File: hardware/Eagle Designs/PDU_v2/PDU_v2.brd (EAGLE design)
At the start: 90.2 x 95.5 mm, 259 parts, among them J1 5037630291, J10 5037630691, J11 UJ31-CH-G1-SMT-TR, J13 5037630291, J14 5037630291, J16 5037630291, J17 5037630291, J18 5037630491, J19 5037630491, J2 5037630291, J20 503182-1852, J21 5037630491, J26 1729128, J29 61300411021, J3 5037630291, J4 5037630291, J5 5037630291, J6 5037630291, J7 5037630491, J8 5037630491, J9 5037630491, M1 BSZ100N06LS3, M2 BSZ100N06LS3, M3 BSZ033NE2LS5, M4 BSZ033NE2LS5, Q1 FDS6375, Q2 FDS6375, Q3 AO4485, SW1 KMR231GLFS, U1 DRV8847PWPR, U11 IRLML2803PBFCT-ND, U12 IRLML2803PBFCT-ND, U13 LT8390EFE#PBF, U14 ATSAME51N19A-AF, U15 INA219BIDR, U16 MAX706RESA+T, U17 MAX16998AAUA+T, U18 ADT7311WTRZ, U19 NTGD1100LT1G, U2 DRV8847PWPR, U20 AO3404A, U21 LT8609A, U22 LT8609A, U23 BC848ALT1G, U3 LTC1477CS8LINEAR_TECHNOLOGY_L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, U4 LTC1477CS8LINEAR_TECHNOLOGY_L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, U5 LTC1477CS8LINEAR_TECHNOLOGY_L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, U6 LTC1477CS8LINEAR_TECHNOLOGY_L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, U7 LTC1477CS8LINEAR_TECHNOLOGY_L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, U8 LT8609A, U9 LTC1477CS8LINEAR_TECHNOLOGY_L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, Y1 CC4V-T1A-32.768KHZ-12.5PF-20P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

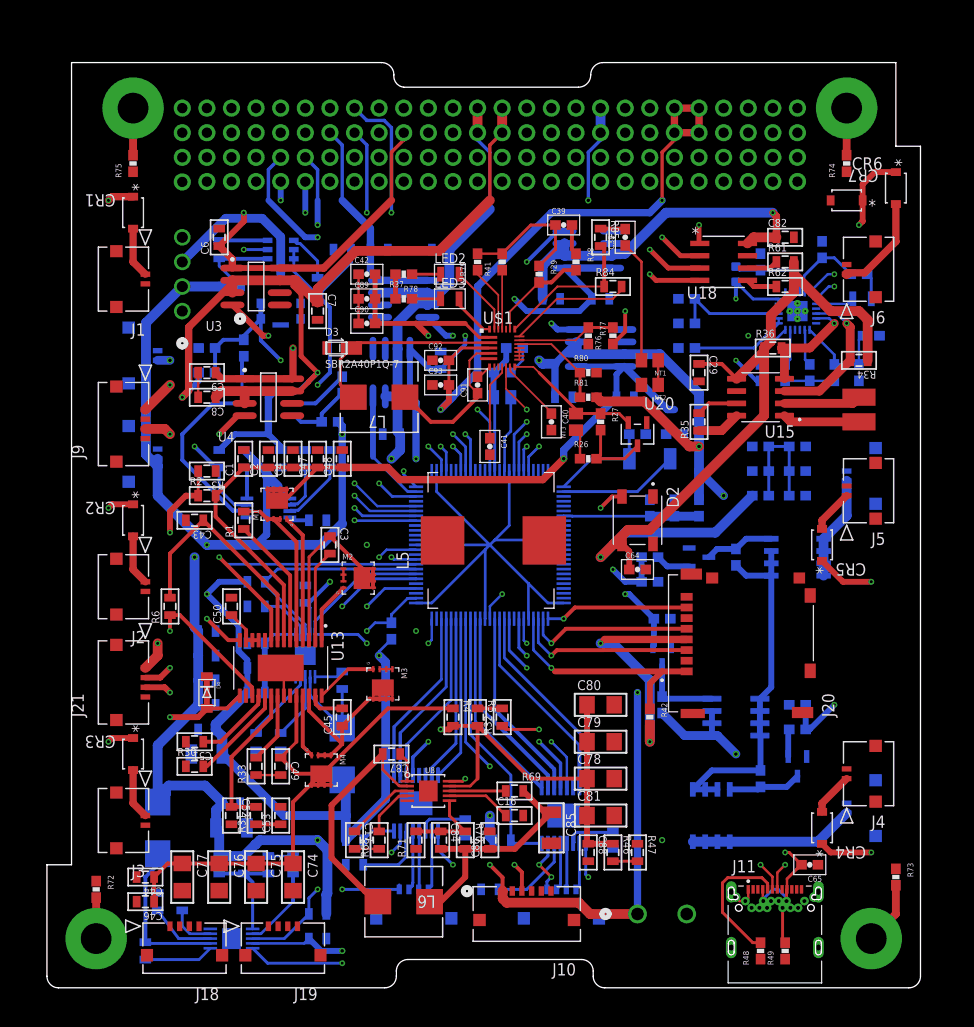
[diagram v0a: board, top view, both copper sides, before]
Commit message: updated PDU v2
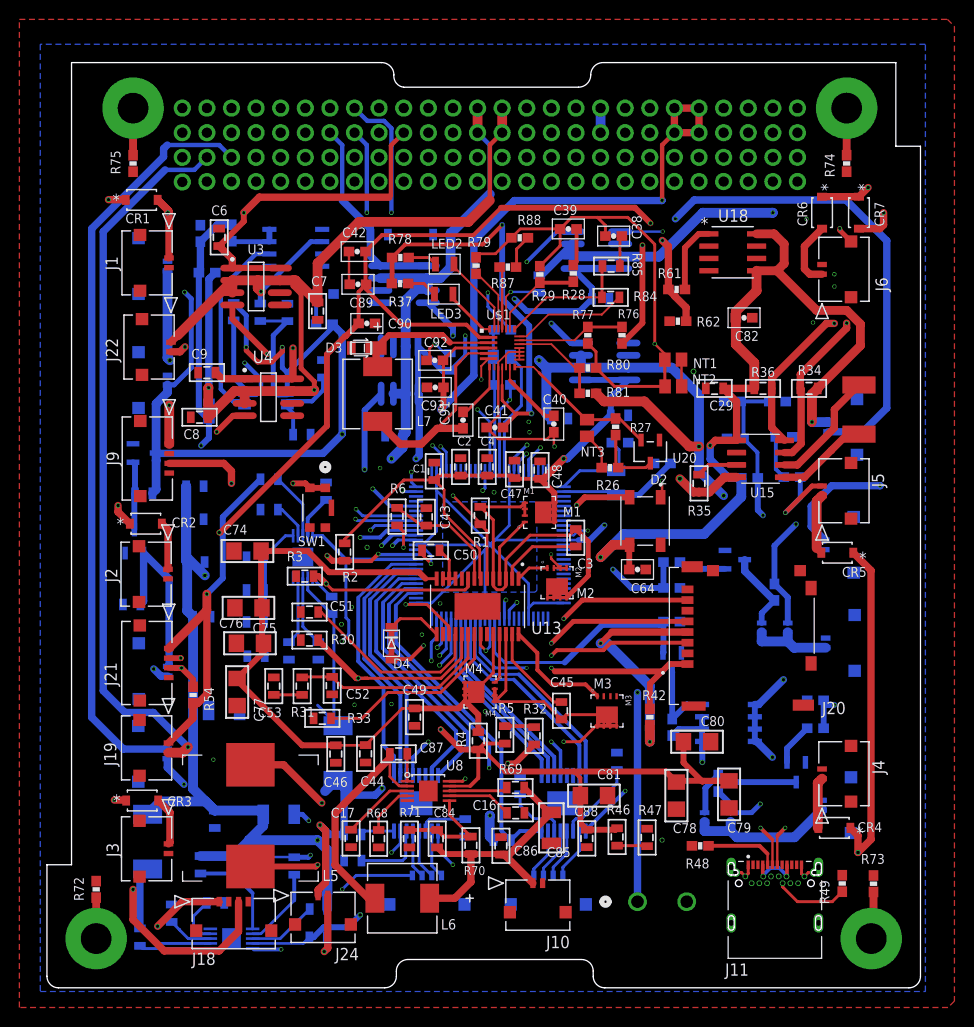
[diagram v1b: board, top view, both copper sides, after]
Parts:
- removed C30, C65: 4.7 uF, HSFL_Main_Library:0603-CAP
- removed C37, C69: 22 uF, HSFL_Main_Library:0603-CAP
- removed C61: 0.1 uF, HSFL_Main_Library:0603-CAP
- removed C66: 47 nF, HSFL_Main_Library:0603-CAP
- removed C67, C68: 10 uF, HSFL_Main_Library:0603-CAP
- removed C70: 1 uF, HSFL_Main_Library:0603-CAP
- removed C83: 0.01 uF, HSFL_Main_Library:0805
- removed J29: 61300411021, Artemis:CONN_61300411021_WRE
- removed L2: 1 uH, Artemis:INDC1608X95N
- removed LED1: LED0805, HSFL_Main_Library:LED_0805
- removed Q1, Q2: FDS6375, Artemis:SOIC127P600X175-8N@1
- removed Q3: AO4485, Artemis:SOIC127P600X175-8N
- removed R39: 316k, HSFL_Main_Library:0603-RES
- removed R40: 110k, HSFL_Main_Library:0603-RES
- removed R41: 84.5k, HSFL_Main_Library:0603-RES
- removed R45, R52: 10k, HSFL_Main_Library:0603-RES
- removed R50: 5.23k, HSFL_Main_Library:0603-RES
- removed R51: 30.1k, HSFL_Main_Library:0603-RES
- removed R53: 383, HSFL_Main_Library:0603-RES
- removed R63: 130k, HSFL_Main_Library:0805
- removed R64: 1M, HSFL_Main_Library:0603-RES
- removed R65: 180k, HSFL_Main_Library:0805
- removed U$6: BQ25883RGER, Artemis:QFN50P400X400X100-25N
- removed U19: NTGD1100LT1G, Artemis:TSOP6_1P70X3P10_ONS
- added J12, J15, J22, J23, J24, J25: 5037630291, Artemis:CON_5037630291
- added R82, R83: 1 M, HSFL_Main_Library:0805
- added R87: 1 M, HSFL_Main_Library:0603-RES
- added R88: 150 k, HSFL_Main_Library:0603-RES
- added U10, U24: AO3404A, Artemis:SOT-23-3L_AOS
- added U25: SI4835DDY-T1-GE3, Artemis:SOIC_DY-T1-GE3_VIS
- added U26, U27: SI3493DDV-T1-GE3, Artemis:6TSOP_VIS
- C1, C2: value 22uF -> 22 uF
- C16, C3, C45, C51, C87: value 0.1uF -> 0.1 uF
- C17, C4: value 1uF -> 1 uF
- C43, C47, C48, C86, C88: value 4.7uF -> 4.7 uF
- C46, C49: value 10uF -> 10 uF
- C50: value 0.47uF -> 0.47 uF
- C52: value 100pF -> 100 pF
- C53: value 4.7nF -> 4.7 nF
- C74, C75, C76, C77, C78, C79, C80, C81: value 33uF -> 33 uF
- C82: device HSFL_Main_Library:0805 -> HSFL_Main_Library:0603-CAP
- C84: value 10pF -> 10 pF
- C85: value 47uF -> 47 uF
- J10: value 5037630691 -> 5037630291; device Artemis:CONN_503763-0691_MOL -> Artemis:CON_5037630291
- J19: value 5037630491 -> 5037630291; device Artemis:CON_5037630491 -> Artemis:CON_5037630291
- L1, L3, L6, L7: value 2.2 uH -> PA4341.222NLT; device Artemis:IND_BOURNS_SRP7030 -> Artemis:IND_222NLT_PUL
- R1: value 4m -> 4 m
- R10, R13, R30, R32, R7: value 10K -> 10 k
- R11, R33, R6, R69, R8: value 100K -> 100 k
- R12, R9: value 4.7K -> 4.7 k
- R14, R22: value 18.2 K -> 18.2 k
- R15: value 301k -> 301 k
- R16, R24: value 47k -> 47 k
- R17, R72, R73, R74, R75: value 1M -> 1 M
- R2: value 390K -> 390 k
- R23: value 180k -> 180 k
- R26, R80, R81: value 1k -> 1 k
- R28, R38, R42, R54, R55, R56, R57, R77, R84, R86: value 10k -> 10 k
- R29: value 40.2k -> 40.2 k
- R3: value 180K -> 180 k
- R31: value 27K -> 27 k
- R34, R36, R43, R44: value 3.3k -> 3.3 k
- R35: value 2m -> 2 m
- R37, R58, R78: value 2k -> 2 k
- R4: value 15m -> 15 m
- R46: value 510K -> 510 k
- R47: value 270K -> 270 k
- R48, R49: value 5.1k -> 5.1 k
- R5: value 130K -> 130 k
- R59: value 100k -> 100 k
- R60: value 62k -> 63.4 k
- R61: value 10k -> 27 k; device HSFL_Main_Library:0805 -> HSFL_Main_Library:0603-RES
- R62: value 10k -> 10 k; device HSFL_Main_Library:0805 -> HSFL_Main_Library:0603-RES
- R66: value 9.09k -> 9.09 k
- R67, R85: value 15k -> 15 k
- R68: value 40.2K -> 40.2 k
- R70: value 1.0M -> 1 M
- R71: value 69.8K -> 69.8 k
- R76: value 27.4k -> 27.4 k
- R79: value 68.1k -> 68.1 k
- U18: value ADT7311WTRZ -> TMP36FSZ
- Y1: value CC4V-T1A-32.768KHZ-12.5PF-20PPM-TA-QC -> ABS07-32.768KHZ-T; device Artemis:XTAL_CC4V-T1A-32.768KHZ-12.5PF-20PPM-TA-QC -> Artemis:XTAL_ABS07-32.768KHZ-T
- moved L5 34.5 mm to (24.0, 25.0), turned to 180 degrees
- moved C74 34.0 mm to (20.7, 45.1), turned to 180 degrees
- moved C75 27.8 mm to (20.8, 39.2), turned to 180 degrees
- moved C44 26.1 mm to (32.9, 24.2), turned to 270 degrees
- moved C3 25.4 mm to (54.6, 46.5)
- moved R6 25.2 mm to (36.1, 48.6)
- moved C46 24.9 mm to (29.8, 24.1), turned to 270 degrees
- moved R1 24.4 mm to (44.7, 48.7)
- moved C76 24.3 mm to (21.0, 35.6), turned to 180 degrees
- moved C43 23.9 mm to (39.2, 48.6), turned to 90 degrees
- moved M1 23.8 mm to (49.2, 47.4), turned to 0 degrees
- moved M3 23.3 mm to (56.2, 30.2)
- moved C45 22.6 mm to (53.1, 28.6)
- moved J19 21.6 mm to (12.5, 25.3), turned to 90 degrees
- moved R54 21.5 mm to (15.1, 30.2), flipped to the top
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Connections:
- net N$60 renamed CCO_0
- net N$62 renamed CCO_1
- removed net BATT_CHRG_DISP: C61.1, R39.1, R40.2, U14.7
- removed net BATT_CHRG_VCC: C41.1, U$1.9
- removed net BUS_EN_VIN: R63.1, R64.2, U19.4
- removed net INH_SW3_COM: J19.3
- removed net INH_SW3_NC: J19.1
- removed net ISET: R41.1, U$1.23
- removed net N$10: LED1.1, R45.2
- removed net N$26: C30.1, U$6.11
- removed net N$30: R53.2, U$6.8
- removed net N$39: C66.1, U$6.12
- removed net N$43: C67.1, L2.1, U$6.21, U$6.22
- removed net N$5: R50.1, R51.2, R52.2, U$6.7
- removed net N$51: C66.2, L2.2, U$6.17, U$6.18
- removed net N$9: LED1.2, U$6.2
- removed net R1/C1: C83.2, R63.2, U19.6
- removed net SPI2_CS0: H1.1.10, U18.4
- removed net SPI2_CT: R61.1, U18.6
- removed net SPI2_D0: H1.1.11, U18.2
- removed net SPI2_D1: H1.1.12, U18.3
- removed net SPI2_INT: R62.1, U18.5
- removed net SPI2_SCLK: H1.1.9, U18.1
- removed net USB_JUMP1: C37.2, C69.2, J29.1, U$6.15, U$6.16
- removed net USB_JUMP_BAT: C68.1, J29.3, U$6.13, U$6.14
- removed net USB_VBUS: C65.2, C70.1, J11.A4, J11.A9, J11.B4, J11.B9, R45.1, R50.2, U$6.23, U14.32
- removed net VIN3: U3.6, U4.6, U5.6, U6.6, U7.6, U9.6
- removed net VL: C42.2, C89.2, C90.2, CR1.1, CR2.1, CR3.1, CR4.1, CR5.1, CR6.1, CR7.1, R76.1, U$1.1
- new net AIN1: H1.1.3, R61.1, R62.2
- new net AIN2: H1.1.4, J19.2
- new net AIN3: H1.1.5, J22.2
- new net AIN4: H1.1.6, J23.2
- new net AIN5: H1.1.7, J24.2
- new net AIN6: H1.1.8, J25.2
- new net N$32: U3.6
- new net N$33: U4.6
- new net N$34: U5.6
- new net N$35: U6.6
- new net N$36: U7.6
- new net N$37: U9.6
- new net N$42: R61.2, U18.1
- new net N$53: R87.1, U$1.23
- new net N$63: R87.2, R88.1
- new net RBF_OUT: J15.2, R83.1, U10.1
- new net VBUS: J11.A4, J11.A9, J11.B4, J11.B9
- net 12V_SW1: now also J10.1; no longer J10.5
- net 5V_BURN: now also U14.37; no longer U14.82
- net 5V_USB_CHRG: now also J12.1
- net BATT_CHRG: no longer J29.4
- net BC_VCC: now also C41.1, U$1.9
- net BURN1_EN: now also U14.96; no longer U14.83
- net BURN2_EN: now also U14.49; no longer U14.84
- net BUS_3V3: now also C82.2, J19.1, J22.1, J23.1, J24.1, J25.1, U18.5, U18.8; no longer R61.2, R62.2
- net BUS_3V3_PG: no longer U14.58
- net BUS_5V: no longer C82.1, U18.8
- net BUS_5V_PG: no longer U14.56
- net BUS_EN: now also U14.60; no longer C83.1, R65.2, U14.57, U19.2, U19.3
- net CUS_SCL: now also U14.35; no longer U$6.5, U14.93
- net CUS_SDA: now also U14.34; no longer U$6.4, U14.94
- net FAULT1: now also U14.53; no longer U14.42
- net GND: now also C82.1, H1.2.9, J10.3, J12.2, J12.3, J12.4, J15.3, J15.4, J19.3, J22.3, J22.4, J23.3, J23.4, J24.3, J24.4, J25.3, J25.4, R62.1, R83.2, U10.2, U18.4, U24.2; no longer C30.2, C37.1, C61.2, C65.1, C67.2, C68.2, C69.1, C70.2, C82.2, J10.6, J19.2, J19.5, J19.6, R40.1, R51.1, R52.1, R53.1, R65.1, U$6.19, U$6.20, U$6.25, U18.7, U19.1
- net GNDA: now also R88.2; no longer R41.2
- net IN1: now also U14.41; no longer U14.35
- net IN2: now also U14.42; no longer U14.36
- net IN3: now also U14.45; no longer U14.41
- net IN4: now also U14.44; no longer U14.40
- net IN5: now also U14.55; no longer U14.44
- net IN6: now also U14.56; no longer U14.45
- net IN7: now also U14.59; no longer U14.48
- net IN8: now also U14.58; no longer U14.47
- net INH_SW1_COM: now also CR1.1, CR2.1, CR3.1, CR4.1, CR5.1, CR6.1, CR7.1, J18.1; no longer J18.3
- net INH_SW1_NC: now also C42.2, C89.2, C90.2, J18.3, R76.1, U$1.1; no longer J18.1
- net LED: now also U14.71; no longer U14.73
- net N$13: now also U25.5, U25.6, U25.7, U25.8, U26.4, U27.4; no longer Q1.1, Q1.2, Q1.3, Q2.1, Q2.2, Q2.3, Q3.5, Q3.6, Q3.7, Q3.8
- net N$15: now also U27.3; no longer Q2.4
- net N$16: now also U25.4; no longer Q3.4
- net N$18: now also U26.3; no longer Q1.4
- net N$20: now also R82.1, U10.3, U24.1; no longer H1.1.32
- net RESET: no longer U19.5
- net SD_CS: now also U14.87; no longer U14.29
- net SD_MISO: now also U14.48; no longer U14.26
- net SD_MOSI: now also U14.46; no longer U14.28
- net SD_SCK: now also U14.47; no longer U14.27
- net SLEEP1: now also U14.40; no longer U14.34
- net SLEEP2: now also U14.54; no longer U14.43
- net SWCLK: now also U14.93; no longer U14.52
- net SWDIO: now also U14.94; no longer U14.54
- net SW_12V_EN1: now also U14.61; no longer U14.59
- net SW_12V_PGOOD: no longer U14.60
- net SW_3V3_EN1: now also U14.64; no longer U14.71
- net SW_3V3_EN2: now also U14.65; no longer U14.70
- net SW_5V_1: no longer J10.3
- net SW_5V_2: no longer J10.1
- net SW_5V_EN1: now also U14.67; no longer U14.75
- net SW_5V_EN2: now also U14.66; no longer U14.74
- net TRQ1: now also U14.43; no longer U14.37
- net TRQ2: now also U14.57; no longer U14.46
- net USB_D+: now also U14.75; no longer U$6.24, U14.95
- net USB_D-: now also U14.74; no longer U$6.1, U14.96
- net VBATT: now also J15.1, R82.2, U24.3, U25.1, U25.2, U25.3; no longer J29.2, Q3.1, Q3.2, Q3.3, R39.2, R64.1
- net VBURN1: now also U26.1, U26.2, U26.5, U26.6; no longer Q1.5, Q1.6, Q1.7, Q1.8
- net VBURN2: now also U27.1, U27.2, U27.5, U27.6; no longer Q2.5, Q2.6, Q2.7, Q2.8
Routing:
- net VL: track 298.8 -> 0.00 mm, vias 8 -> 0
- net INH_SW1_COM: track 0.00 -> 278.2 mm, vias 0 -> 6
- net INH_SW1_NC: track 0.00 -> 158.2 mm, vias 0 -> 4
- net AIN5: track 0.00 -> 124.6 mm, vias 0 -> 1
- net AIN6: track 0.00 -> 96.3 mm, vias 0 -> 1
- net SW_5V_1: track 108.8 -> 20.8 mm, vias 1 -> 0
- net SOLAR_IN1: track 9.74 -> 94.5 mm, vias 0 -> 3
- net AIN4: track 0.00 -> 78.6 mm
- net AIN2: track 0.00 -> 74.7 mm, vias 0 -> 1
- net VBATT: track 426.0 -> 351.6 mm, vias 10 -> 11
- net N$41: track 19.4 -> 80.7 mm, vias 0 -> 2
- net USB_VBUS: track 59.2 -> 0.00 mm, vias 2 -> 0
- net AIN1: track 0.00 -> 58.9 mm, vias 0 -> 1
- net GNDA: track 33.2 -> 90.6 mm, vias 1 -> 2
- net BUS_EN: track 114.4 -> 58.0 mm, vias 3 -> 2
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- added copper zone on layer 1, net GND
- added copper zone on layer 15, net GND
- added copper zone on layer 16, net GND
- added copper zone on layer 2, net GND
- added copper zone on layer 16, net VDD
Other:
- board text added: "5V BUS"
- board text added: "5V SW 3"
- board text added: "Burn 1"
- board text added: "Burn 2"
- board text added: "Burn Wire Circuit"
- board text added: "C:/Users/kelly/Downloads/artemissssssssssss.bmp"
- board text added: "HB1"
- board text added: "HB1 Torque"
- board text added: "HB2"
- board text added: "HB2 Torque"
- board text added: "Heater"
- board text added: "M1"
- board text added: "M2"
- board text added: "M3"
- board text added: "M4"
- board text added: "TPS AIN6"
- board text added: "USB Charge"
- board text added: "VBATT SW 1"
